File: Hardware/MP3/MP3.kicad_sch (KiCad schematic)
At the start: 1 part, among them J1 Conn_02x20_Odd_Even

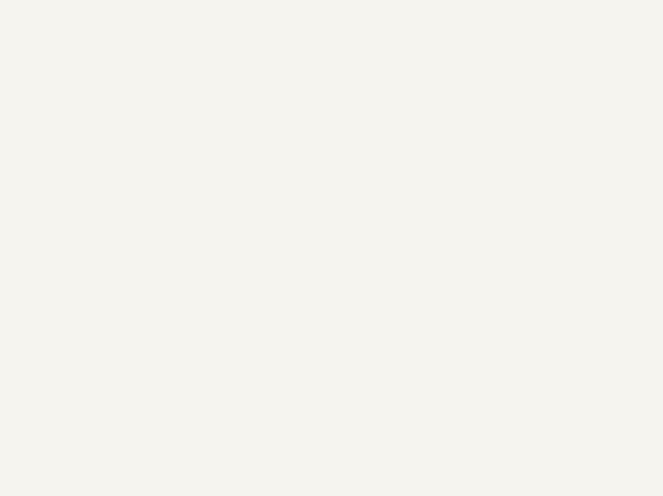
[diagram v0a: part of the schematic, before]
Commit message: Schematic notes
- notes regarding schematic layout and included ICs
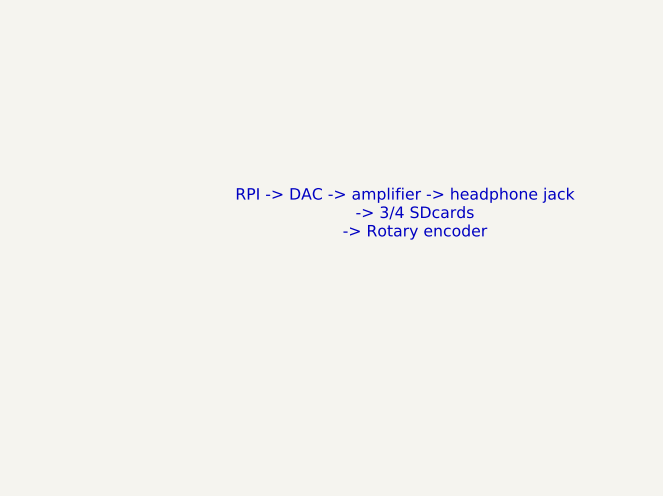
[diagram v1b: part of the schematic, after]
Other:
- note added: "RPI -> DAC -> amplifier -> headphone jack -> 3/4 SDcards -> Rotary encoder"
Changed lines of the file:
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@@
 	(generator_version "9.0")
 	(paper "A4")
+	(text "RPI -> DAC -> amplifier -> headphone jack\n	-> 3/4 SDcards\n	-> Rotary encoder\n"
+		(exclude_from_sim no)
+		(at 166.116 47.498 0)
+		(effects
+			(font
+				(size 1.27 1.27)
+			)
+		)
+	)
 	(text "SPI pinouts can be unreliable, double triple check to make sure that they are correct"
 		(exclude_from_sim no)
